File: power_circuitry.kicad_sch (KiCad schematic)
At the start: 16 parts, among them J1 Power_Input, Q1 SI3127DV-T1-GE3, U1 AP63203WU-7

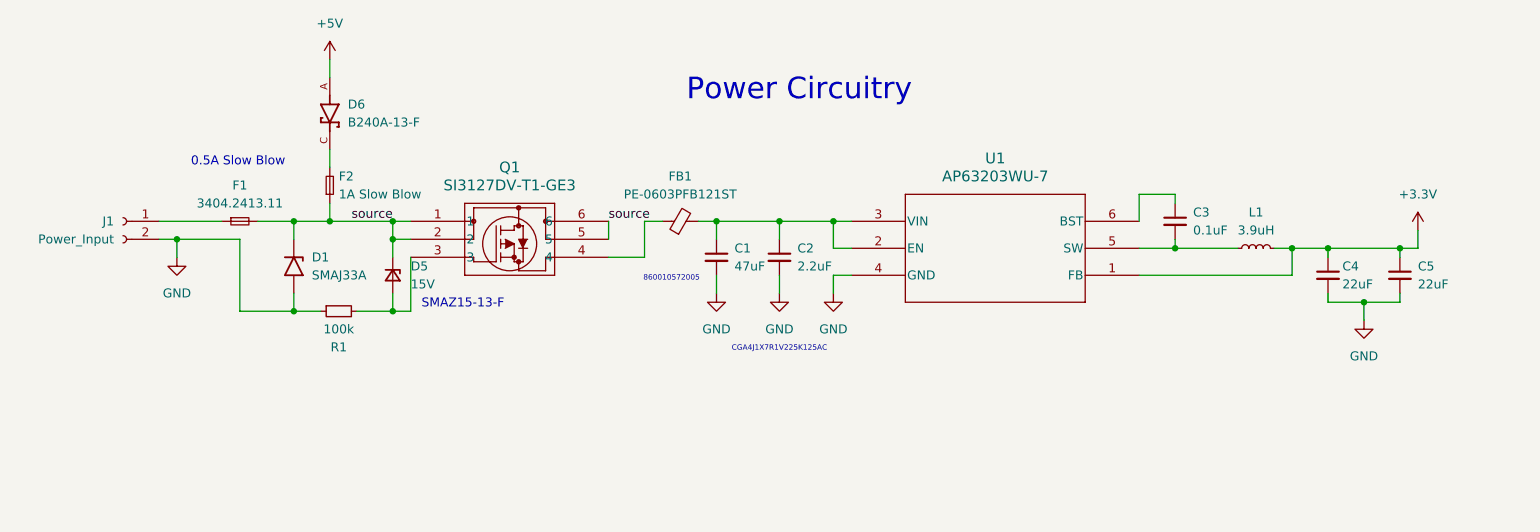
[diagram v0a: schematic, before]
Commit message: Rev A PCB Ordered
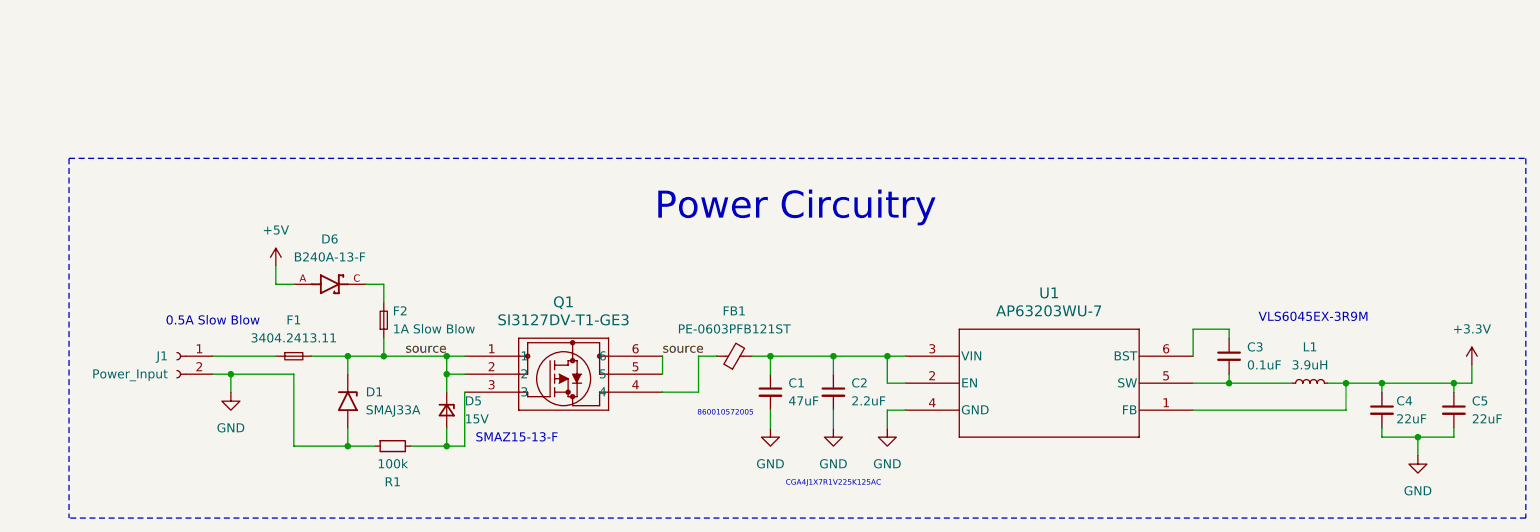
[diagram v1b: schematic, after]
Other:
- note added: "VLS6045EX-3R9M"
- company: (none) -> FrostByte Solutions
- title: (none) -> FrostByte IR Camera Interface Board
- moved on the sheet: C1, C2, C3, C4, C5, D1, D5, D6, F1, F2, FB1, J1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
